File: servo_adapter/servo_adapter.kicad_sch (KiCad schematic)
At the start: 10 parts, among them J1 T4140012081-000, Q1 MUN5233, Q2 MUN5233, Q3 MUN5233, Q4 MUN5233

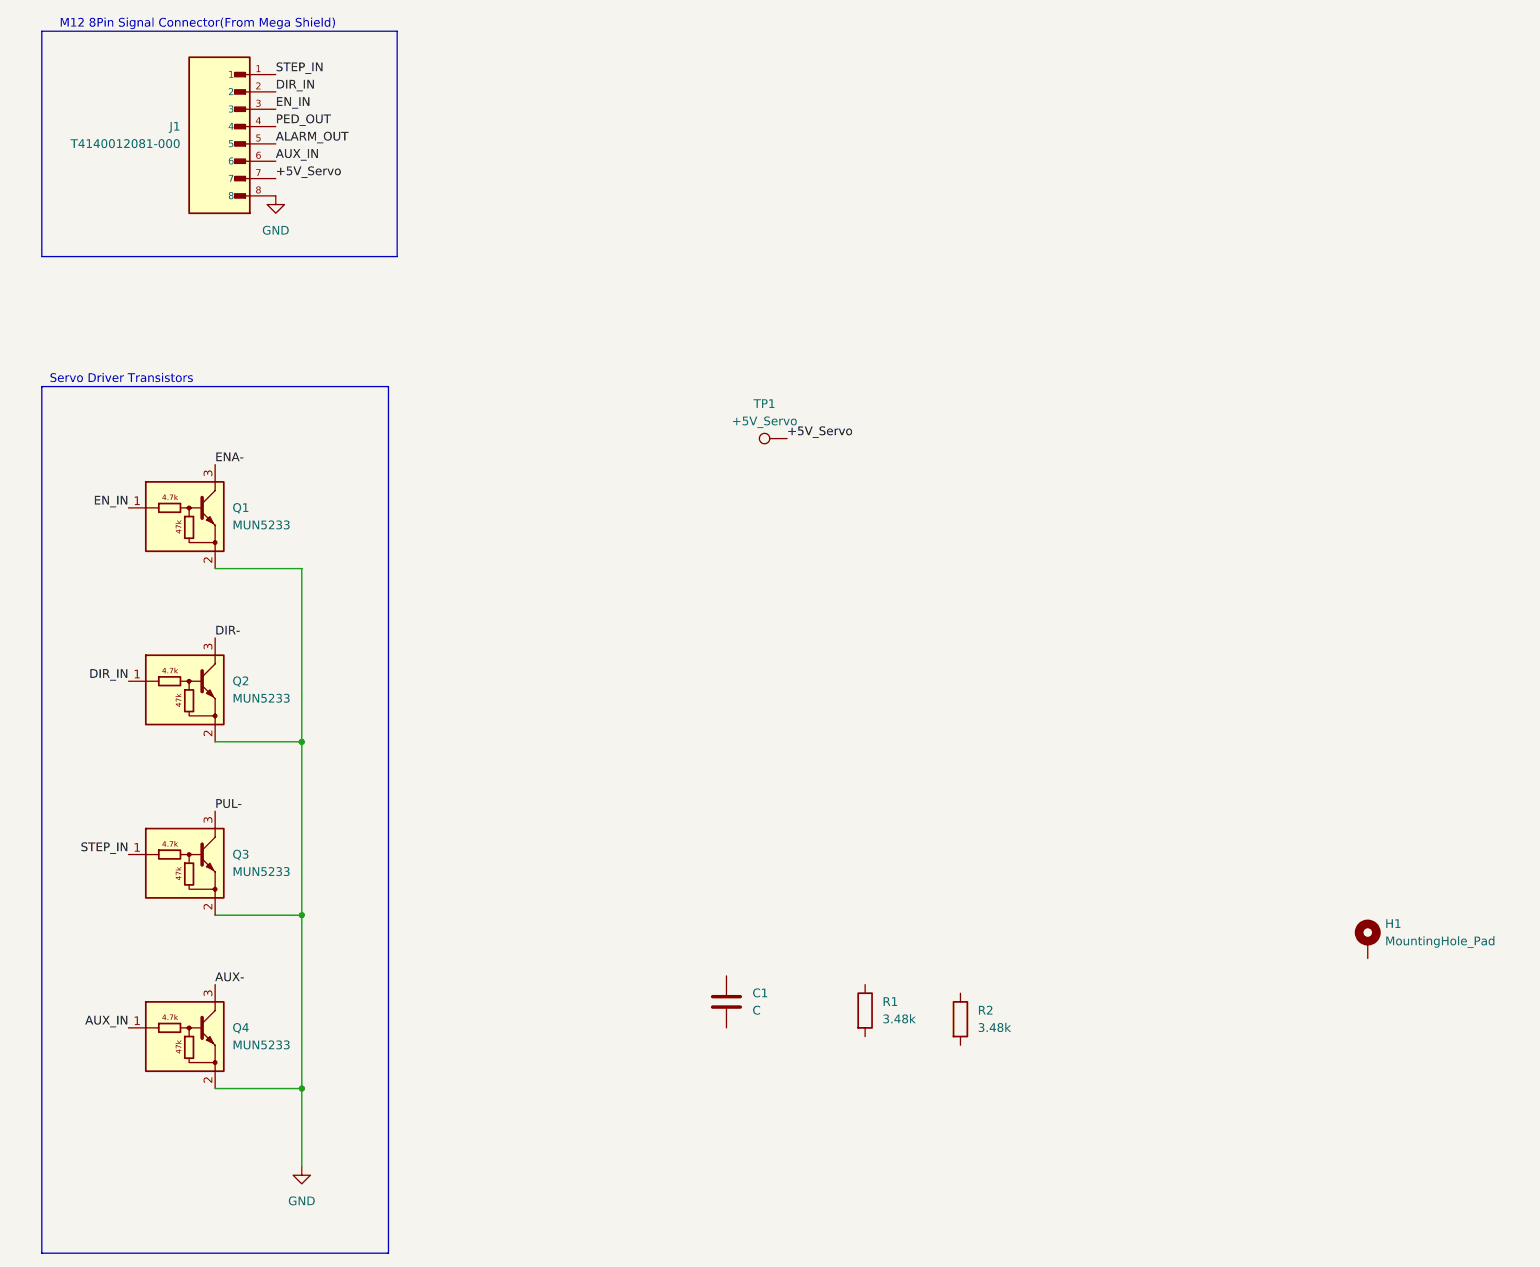
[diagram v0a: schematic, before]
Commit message: Added the 10pin female socket (adapter --> servo motor) and labels for each of the pins along with passive components.
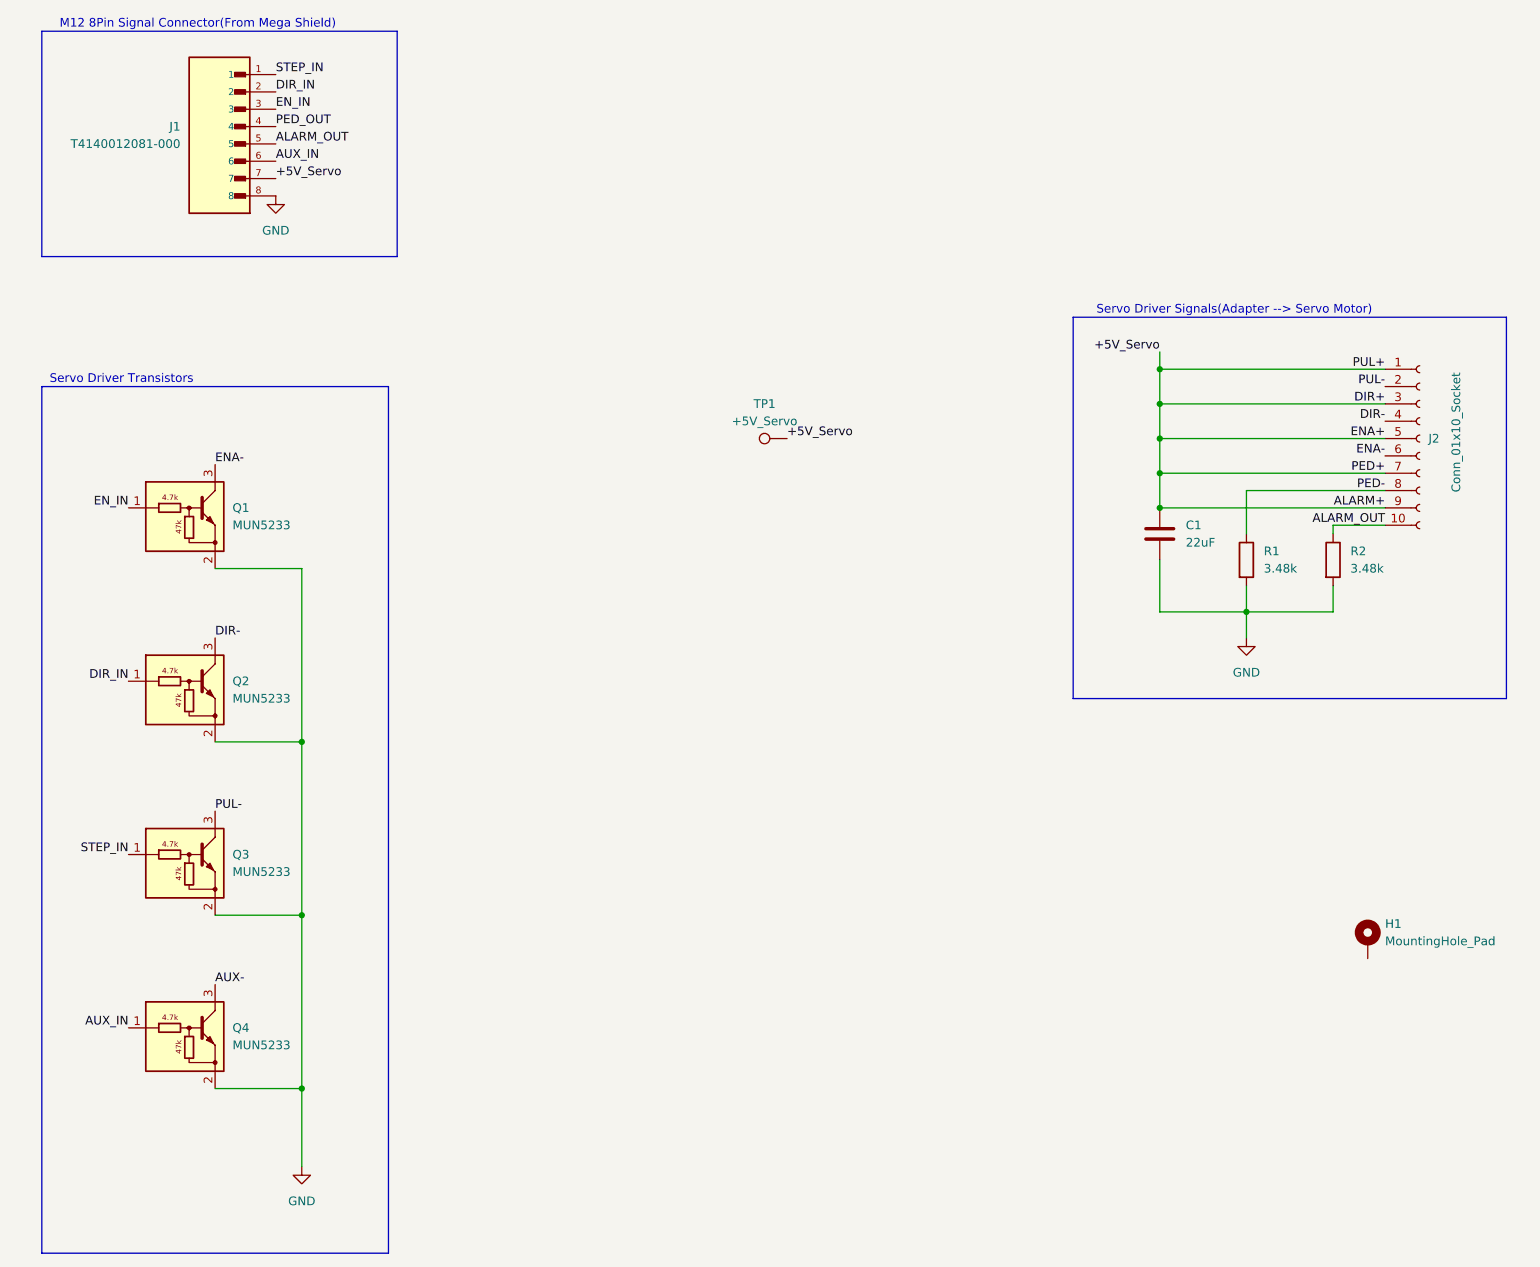
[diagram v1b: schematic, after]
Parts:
- added J2: Conn_01x10_Socket, symbol Connector:Conn_01x10_Socket
- C1: value C -> 22uF
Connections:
- net +5V_Servo: now also C1.1, J2.1 (Pin_1), J2.3 (Pin_3), J2.5 (Pin_5), J2.7 (Pin_7), J2.9 (Pin_9)
- net ALARM_OUT: now also R2.1, J2.10 (Pin_10)
- net DIR-: now also J2.4 (Pin_4)
- net ENA-: now also J2.6 (Pin_6)
- net GND: now also C1.2, R1.2, R2.2
- net PUL-: now also J2.2 (Pin_2)
- net PED-: now reaches R1.1
- net PED-: now also J2.8 (Pin_8)
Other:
- note added: "Servo Driver Signals(Adapter --> Servo Motor)"
- moved on the sheet: C1, R1, R2
